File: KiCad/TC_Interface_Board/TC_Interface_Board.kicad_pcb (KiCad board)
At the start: 2 copper layers, 68.9 x 121.6 mm, 30 parts, among them J1 Conn_01x05, J1_24V1 JST_VH_01x04, J1_CN1 JST_VH_01x03, J2 Conn_01x05, J2_CN1 JST_VH_01x02, J3 Conn_01x05, J3_CN1 JST_VH_01x02, J4 Conn_01x05, J5 Conn_01x05, J6 Conn_01x05, J7 Conn_01x05, J8 Conn_01x05, Q1 DTC143E, Q2 DTC143E, U1 MC34063AP

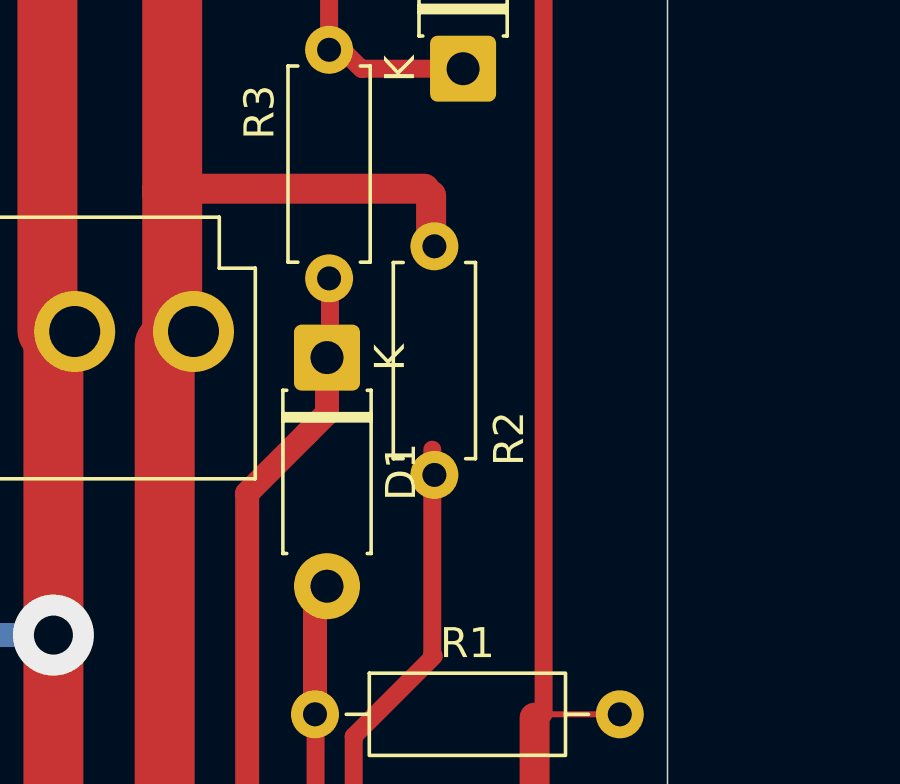
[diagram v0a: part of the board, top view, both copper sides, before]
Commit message: UPDATE
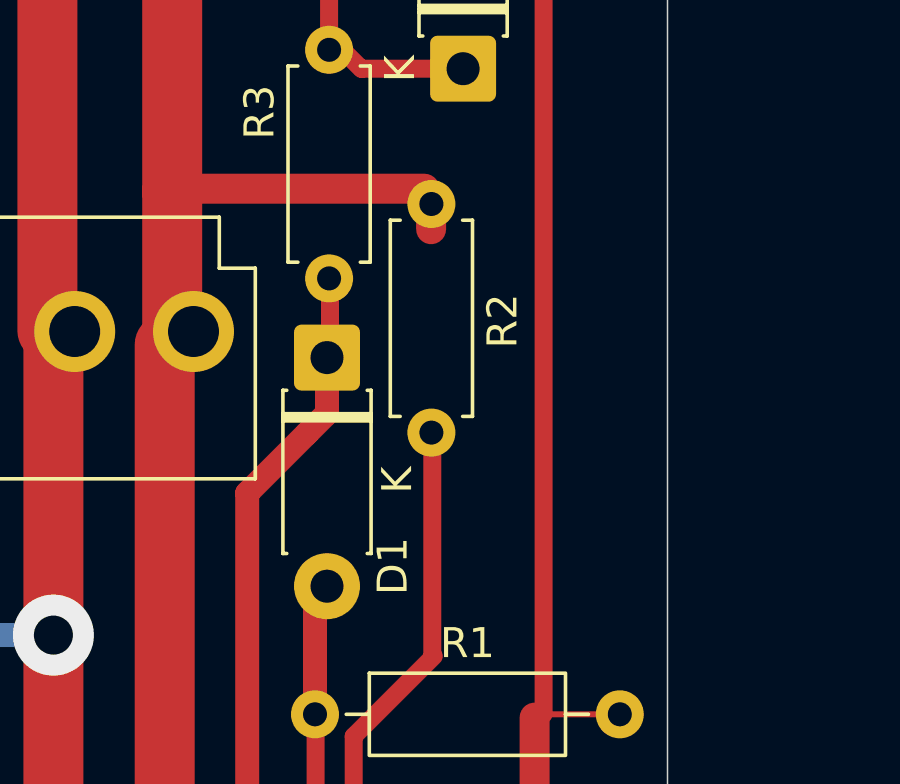
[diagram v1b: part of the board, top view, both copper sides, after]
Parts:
- moved R2 9.03 mm to (169.8, 84.8), turned to -90 degrees
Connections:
- C1 pad 1: Net-(D3-K) -> /MC34063_TC
- C2 pad 1: /MC34063_TC -> Net-(D5-K)
- D5 pad 1: /MC34063_TC -> Net-(D5-K)
- R3 pad 1: Net-(Q1-B) -> /CMD_IN
- R5 pad 2: /MC34063_TC -> Net-(D5-K)
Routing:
- net (no net): track 105.5 -> 78.6 mm
- net Net-(Q1-B): track 0.00 -> 26.9 mm
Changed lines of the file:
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@@
 	(net 19 "/Q2_BASE")
 	(net 20 "Net-(Q1-B)")
+	(net 21 "Net-(D5-K)")
 	(footprint "Connector_JST:JST_VH_B5P-VH-B_1x05_P3.96mm_Vertical"
 		(layer "F.Cu")
@@
 	(footprint "Resistor_THT:R_Axial_DIN0207_L6.3mm_D2.5mm_P7.62mm_Horizontal"
 		(layer "F.Cu")
-		(at 169.92 93.83 90)
+		(at 169.82 84.8 -90)
 		(descr "Resistor, Axial_DIN0207 series, Axial, Horizontal, pin pitch=7.62mm, 0.25W = 1/4W, length*diameter=6.3*2.5mm^2, http://cdn-reichelt.de/documents/datenblatt/B400/1_4W%23YAG.pdf")
 		(tags "Resistor Axial_DIN0207 series Axial Horizontal pin pitch 7.62mm 0.25W = 1/4W length 6.3mm diameter 2.5mm")
 		(property "Reference" "R2"
-			(at 1.21 2.49 90)
+			(at 3.9 -2.37 90)
 			(layer "F.SilkS")
 			(effects
@@
 		(attr through_hole)
 		(fp_line
-			(start 7.08 -1.37)
-			(end 7.08 -1.04)
+			(start 0.54 1.37)
+			(end 7.08 1.37)
 			(stroke
 				(width 0.12)
@@
 		)
 		(fp_line
-			(start 0.54 -1.37)
-			(end 7.08 -1.37)
+			(start 7.08 1.37)
+			(end 7.08 1.04)
 			(stroke
 				(width 0.12)
@@
 		)
 		(fp_line
-			(start 0.54 -1.04)
-			(end 0.54 -1.37)
+			(start 0.54 1.04)
+			(end 0.54 1.37)
 			(stroke
 				(width 0.12)
@@
 		)
 		(fp_line
-			(start 0.54 1.04)
-			(end 0.54 1.37)
+			(start 0.54 -1.04)
+			(end 0.54 -1.37)
 			(stroke
 				(width 0.12)
@@
 		)
 		(fp_line
-			(start 7.08 1.37)
-			(end 7.08 1.04)
+			(start 0.54 -1.37)
+			(end 7.08 -1.37)
 			(stroke
 				(width 0.12)
@@
 		)
 		(fp_line
-			(start 0.54 1.37)
-			(end 7.08 1.37)
+			(start 7.08 -1.37)
+			(end 7.08 -1.04)
 			(stroke
 				(width 0.12)
@@
 		)
 		(fp_line
-			(start 7.62 0)
-			(end 6.96 0)
+			(start 0 0)
+			(end 0.66 0)
 			(stroke
 				(width 0.1)
@@
 		)
 		(fp_line
-			(start 0 0)
-			(end 0.66 0)
+			(start 7.62 0)
+			(end 6.96 0)
 			(stroke
 				(width 0.1)
@@
 		)
 		(pad "1" thru_hole circle
-			(at 0 0 90)
+			(at 0 0 270)
 			(size 1.6 1.6)
 			(drill 0.8)
@@
 		)
 		(pad "2" thru_hole circle
-			(at 7.62 0 90)
+			(at 7.62 0 270)
 			(size 1.6 1.6)
 			(drill 0.8)
@@
 			(layers "*.Cu" "*.Mask")
 			(remove_unused_layers no)
-			(net 20 "Net-(Q1-B)")
+			(net 12 "/CMD_IN")
 			(pintype "passive")
 		)
@@
 		(tags "Diode DO-41_SOD81 series Axial Horizontal pin pitch 7.62mm  length 5.2mm diameter 2.7mm")
 		(property "Reference" "D1"
-			(at 3.81 -2.47 270)
+			(at 6.95 -2.19 270)
 			(layer "F.SilkS")
 			(effects
@@
 		)
 		(fp_text user "K"
-			(at 0 -2.1 270)
+			(at 4.08 -2.34 270)
 			(layer "F.SilkS")
 			(effects
@@
 			(remove_unused_layers no)
 			(roundrect_rratio 0.15625)
-			(net 8 "/MC34063_TC")
+			(net 21 "Net-(D5-K)")
 			(pintype "passive")
 		)
@@
 			(layers "*.Cu" "*.Mask")
 			(remove_unused_layers no)
-			(net 8 "/MC34063_TC")
+			(net 21 "Net-(D5-K)")
 			(pintype "passive")
 		)
@@
 			(remove_unused_layers no)
 			(roundrect_rratio 0.15625)
-			(net 17 "Net-(D3-K)")
+			(net 8 "/MC34063_TC")
 			(pintype "passive")
 		)
@@
 			(remove_unused_layers no)
 			(roundrect_rratio 0.15625)
-			(net 8 "/MC34063_TC")
+			(net 21 "Net-(D5-K)")
 			(pinfunction "K")
 			(pintype "passive")
@@
 	)
 	(segment
-		(start 169.9006 99.8728)
-		(end 169.8498 99.822)
-		(width 0.2)
-		(layer "F.Cu")
-		(net 0)
-	)
-	(segment
 		(start 167.321 42.4039)
 		(end 167.0861 42.169)
@@
 	)
 	(segment
-		(start 167.2082 111.221)
-		(end 167.23 111.221)
-		(width 0.2)
-		(layer "F.Cu")
-		(net 0)
-	)
-	(segment
 		(start 156.46 51.44)
 		(end 156.46 45.463572)
@@
 	)
 	(segment
-		(start 167.2082 117.5882)
-		(end 167.2082 111.221)
-		(width 0.6)
-		(layer "F.Cu")
-		(net 0)
-	)
-	(segment
-		(start 167.23 102.5434)
-		(end 169.9006 99.8728)
-		(width 0.6)
-		(layer "F.Cu")
-		(net 0)
-	)
-	(segment
 		(start 150.12 37.25)
 		(end 152.54 39.67)
@@
 	)
 	(segment
-		(start 167.23 110.62)
-		(end 167.23 102.5434)
-		(width 0.6)
-		(layer "F.Cu")
-		(net 0)
-	)
-	(segment
 		(start 167.5 80.29)
 		(end 167.49 80.3)
@@
 	)
 	(segment
-		(start 168.46 118.84)
-		(end 167.2082 117.5882)
-		(width 0.6)
-		(layer "F.Cu")
-		(net 0)
-	)
-	(segment
 		(start 159.136428 63.9)
 		(end 160.386428 62.65)
@@
 	)
 	(segment
-		(start 169.8498 99.822)
-		(end 169.8498 92.9894)
-		(width 0.6)
-		(layer "F.Cu")
-		(net 0)
-	)
-	(segment
 		(start 163.87 57.08)
 		(end 159.49 52.7)
@@
 		(net 19)
 	)
+	(segment
+		(start 169.9006 99.8728)
+		(end 169.8498 99.822)
+		(width 0.2)
+		(layer "F.Cu")
+		(net 20)
+	)
+	(segment
+		(start 167.2082 111.221)
+		(end 167.23 111.221)
+		(width 0.2)
+		(layer "F.Cu")
+		(net 20)
+	)
+	(segment
+		(start 167.2082 117.5882)
+		(end 167.2082 111.221)
+		(width 0.6)
+		(layer "F.Cu")
+		(net 20)
+	)
+	(segment
+		(start 167.23 102.5434)
+		(end 169.9006 99.8728)
+		(width 0.6)
+		(layer "F.Cu")
+		(net 20)
+	)
+	(segment
+		(start 167.23 110.62)
+		(end 167.23 102.5434)
+		(width 0.6)
+		(layer "F.Cu")
+		(net 20)
+	)
+	(segment
+		(start 168.46 118.84)
+		(end 167.2082 117.5882)
+		(width 0.6)
+		(layer "F.Cu")
+		(net 20)
+	)
+	(segment
+		(start 169.8498 99.822)
+		(end 169.8498 92.9894)
+		(width 0.6)
+		(layer "F.Cu")
+		(net 20)
+	)
 	(embedded_fonts no)
